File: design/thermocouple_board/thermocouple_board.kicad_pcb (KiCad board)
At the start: 2 copper layers, 73.9 x 56.6 mm, 68 parts, among them J1 Prog Conn, J2 CAN Conn, J3 CAN Ext Conn, J4 Thermocouple conn, J5 Thermocouple conn, J6 Thermocouple conn, J7 Thermocouple conn, U1 PIC18LF26K83, U2 MCP2562, U3 AP2120N-3.3TRG1, U4 MAX31855KASA, U5 MAX31855KASA, U6 MAX31855KASA, U7 MAX31855KASA, Y1 12 MHz

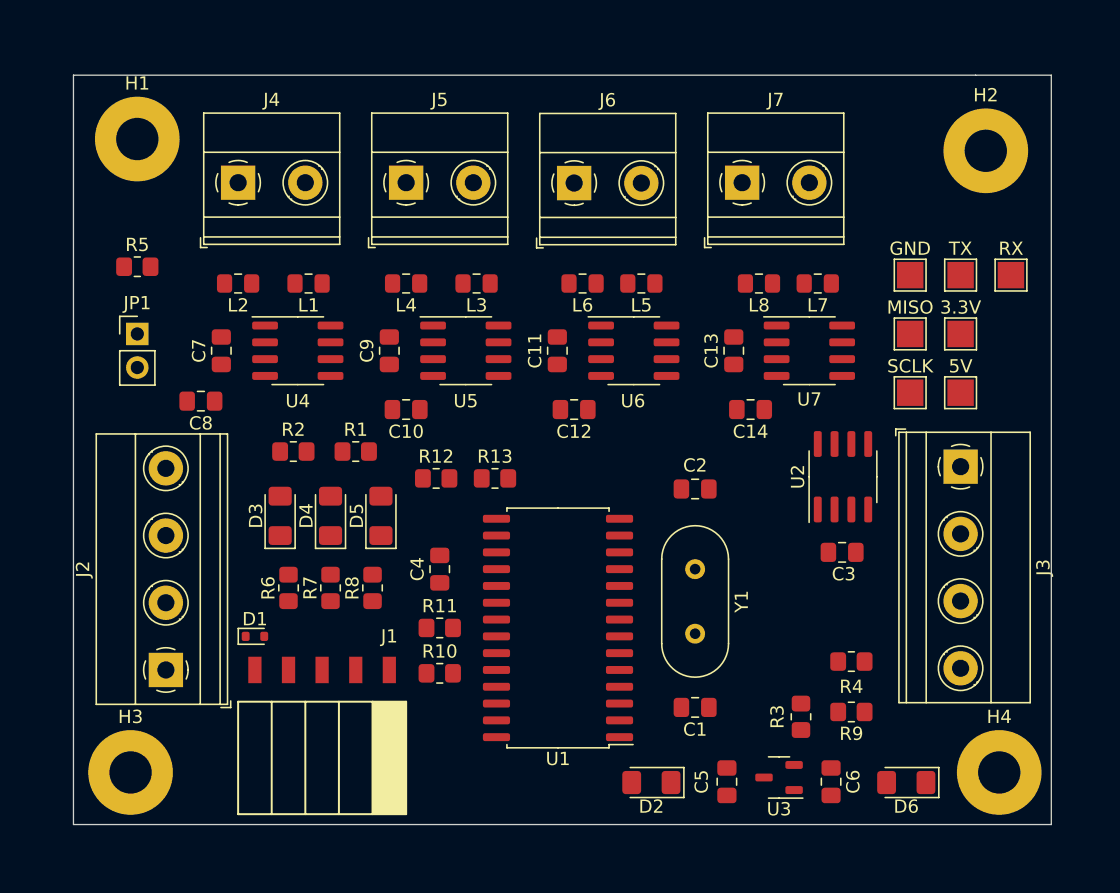
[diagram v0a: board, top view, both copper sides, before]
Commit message: Finished routing, still need to add logo
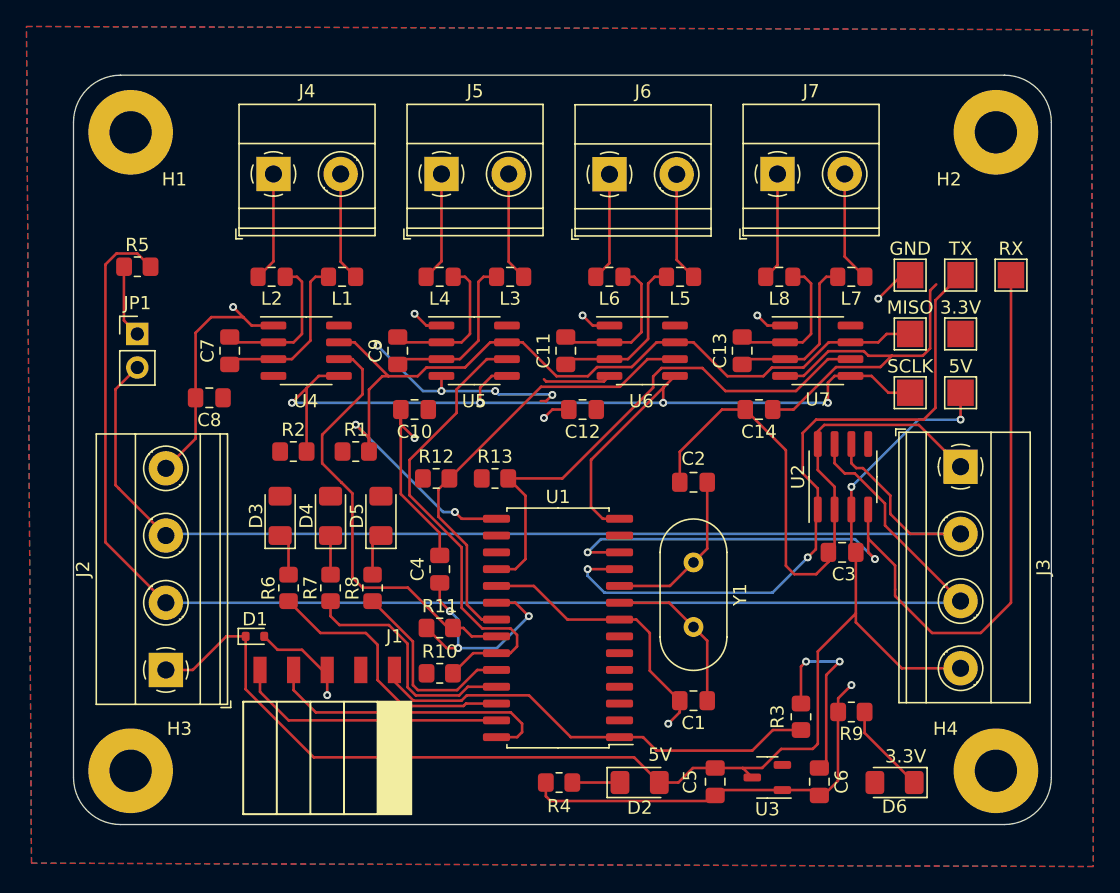
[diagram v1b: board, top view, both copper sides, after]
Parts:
- moved R4 23.9 mm to (137.8, 124.7), turned to 180 degrees
- moved L5 2.97 mm to (146.9, 86.5)
- moved J7 2.75 mm to (154.3, 78.7)
- moved J4 2.75 mm to (116.2, 78.7)
- moved J5 2.75 mm to (128.9, 78.7)
- moved J6 2.75 mm to (141.6, 78.7)
- moved L1 2.58 mm to (121.4, 86.5)
- moved L2 2.58 mm to (116.1, 86.5)
- moved L4 2.58 mm to (128.8, 86.5)
- moved L3 2.58 mm to (134.1, 86.5)
- moved L7 2.58 mm to (159.9, 86.5)
- moved L6 2.09 mm to (141.6, 86.5)
- moved L8 1.62 mm to (154.4, 86.5)
- moved H2 1.59 mm to (170.8, 75.6)
- moved C5 0.89 mm to (149.6, 124.7)
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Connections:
- J3 pad 1: +5V -> GND
- J3 pad 2: /CANH -> /CANL
- J3 pad 3: /CANL -> /CANH
- J3 pad 4: GND -> +5V
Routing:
- net GND: track 0.00 -> 155.6 mm, vias 0 -> 10
- net /CANH: track 0.00 -> 108.0 mm
- net +5V: track 0.00 -> 102.7 mm, vias 0 -> 2
- net /CANL: track 0.00 -> 87.8 mm
- net +3.3V: track 0.00 -> 82.5 mm, vias 0 -> 9
- net SCLK: track 0.00 -> 77.9 mm, vias 0 -> 4
- net MISO: track 0.00 -> 72.4 mm, vias 0 -> 2
- net /CAN_RX: track 0.00 -> 69.9 mm, vias 0 -> 2
- net /CAN_TX: track 0.00 -> 53.0 mm, vias 0 -> 2
- net /CS4: track 0.00 -> 40.7 mm
- net /CS1: track 0.00 -> 36.0 mm
- net /~{MCLR}: track 0.00 -> 34.8 mm
- net /CS3: track 0.00 -> 34.3 mm
- net /CS2: track 0.00 -> 32.8 mm
- net /ICSPDAT: track 0.00 -> 22.6 mm
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- added copper zone on F.Cu, net +3.3V
- added copper zone on B.Cu, net GND
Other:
- outline, holes or cut-outs redrawn
- board text added: "3.3V"
- board text added: "5V"
